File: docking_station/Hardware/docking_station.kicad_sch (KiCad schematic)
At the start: 86 parts, among them IC1 VOM1271T, IC2 VOM1271T, IC3 VOM1271T, IC4 VOM1271T, IC5 VOM1271T, J1 WAGO, J2 XT60, J3 Conn_01x05_Pin, J5 SUPPLY+, J6 SUPPLY-, K1 RELPOL R40N-3021-85-1024, Q1 SIDR392DP-T1-GE3, Q10 2N7002K, Q11 2N7002K, Q12 2N7002K, Q2 SIDR392DP-T1-GE3, Q3 SIDR392DP-T1-GE3, Q4 SIDR392DP-T1-GE3, Q5 SIDR392DP-T1-GE3, Q6 SIDR392DP-T1-GE3, Q7 SIDR392DP-T1-GE3, Q8 SIDR392DP-T1-GE3, Q9 SIDR392DP-T1-GE3, U1 LTC4357MS8, U2 ACS712xLCTR-20A, U3 L78L05AB, U4 LMV321IYLT, U5 MCP6561T-E/OT, U6 MCP6561T-E/OT

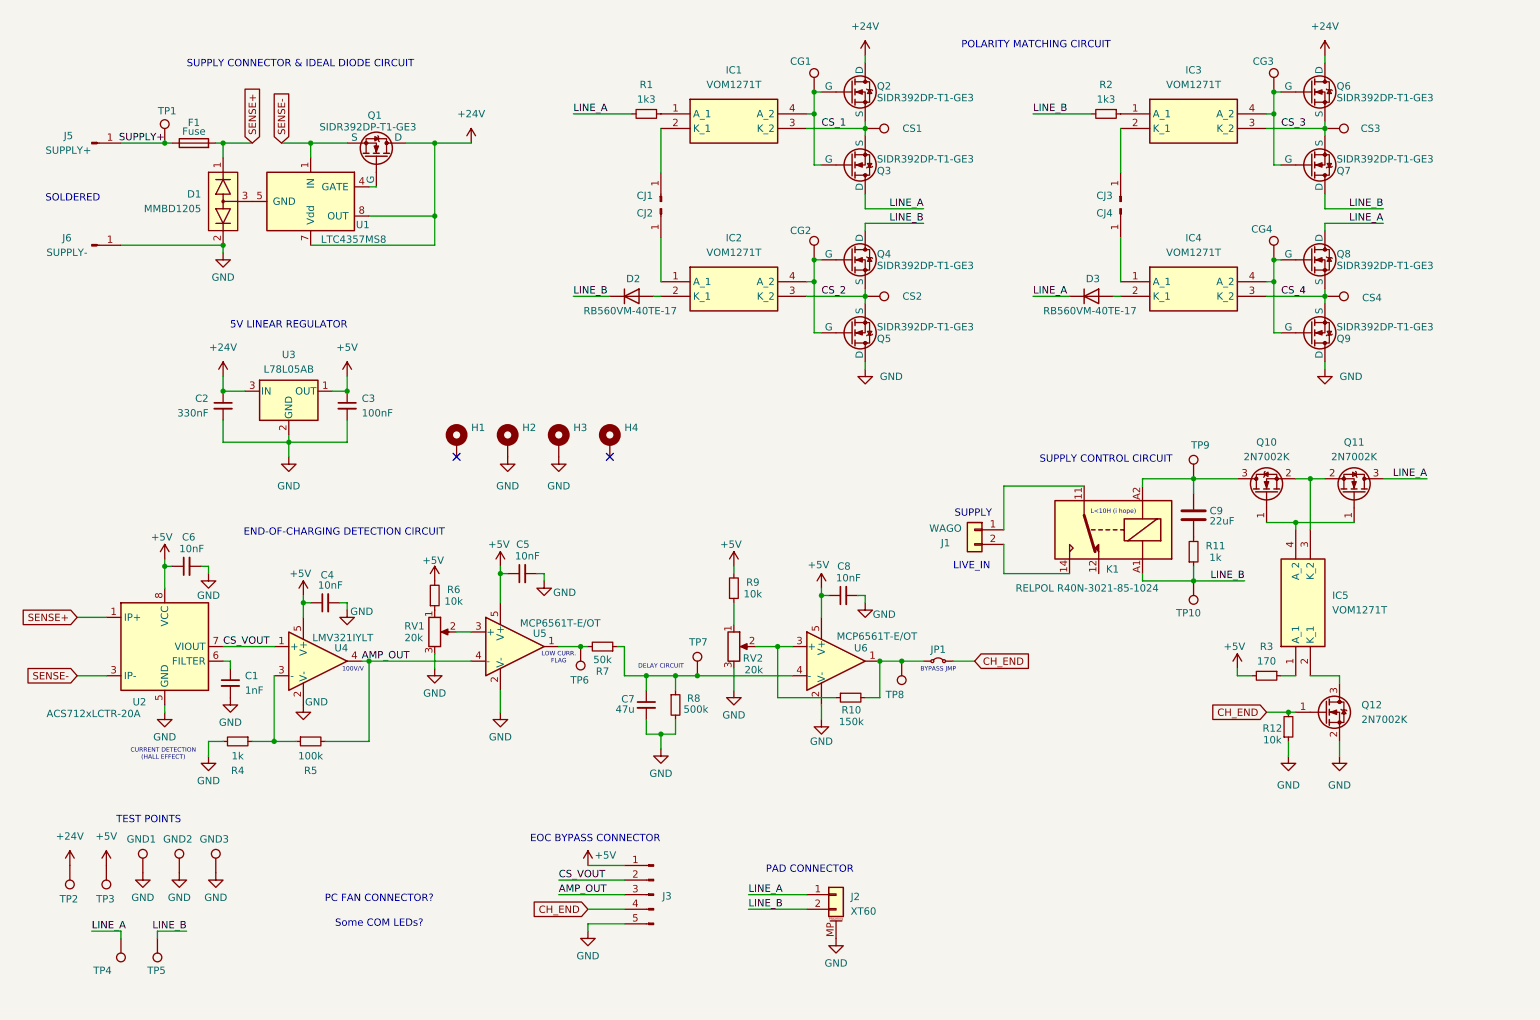
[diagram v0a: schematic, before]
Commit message: Readability update begin
Added LEDs
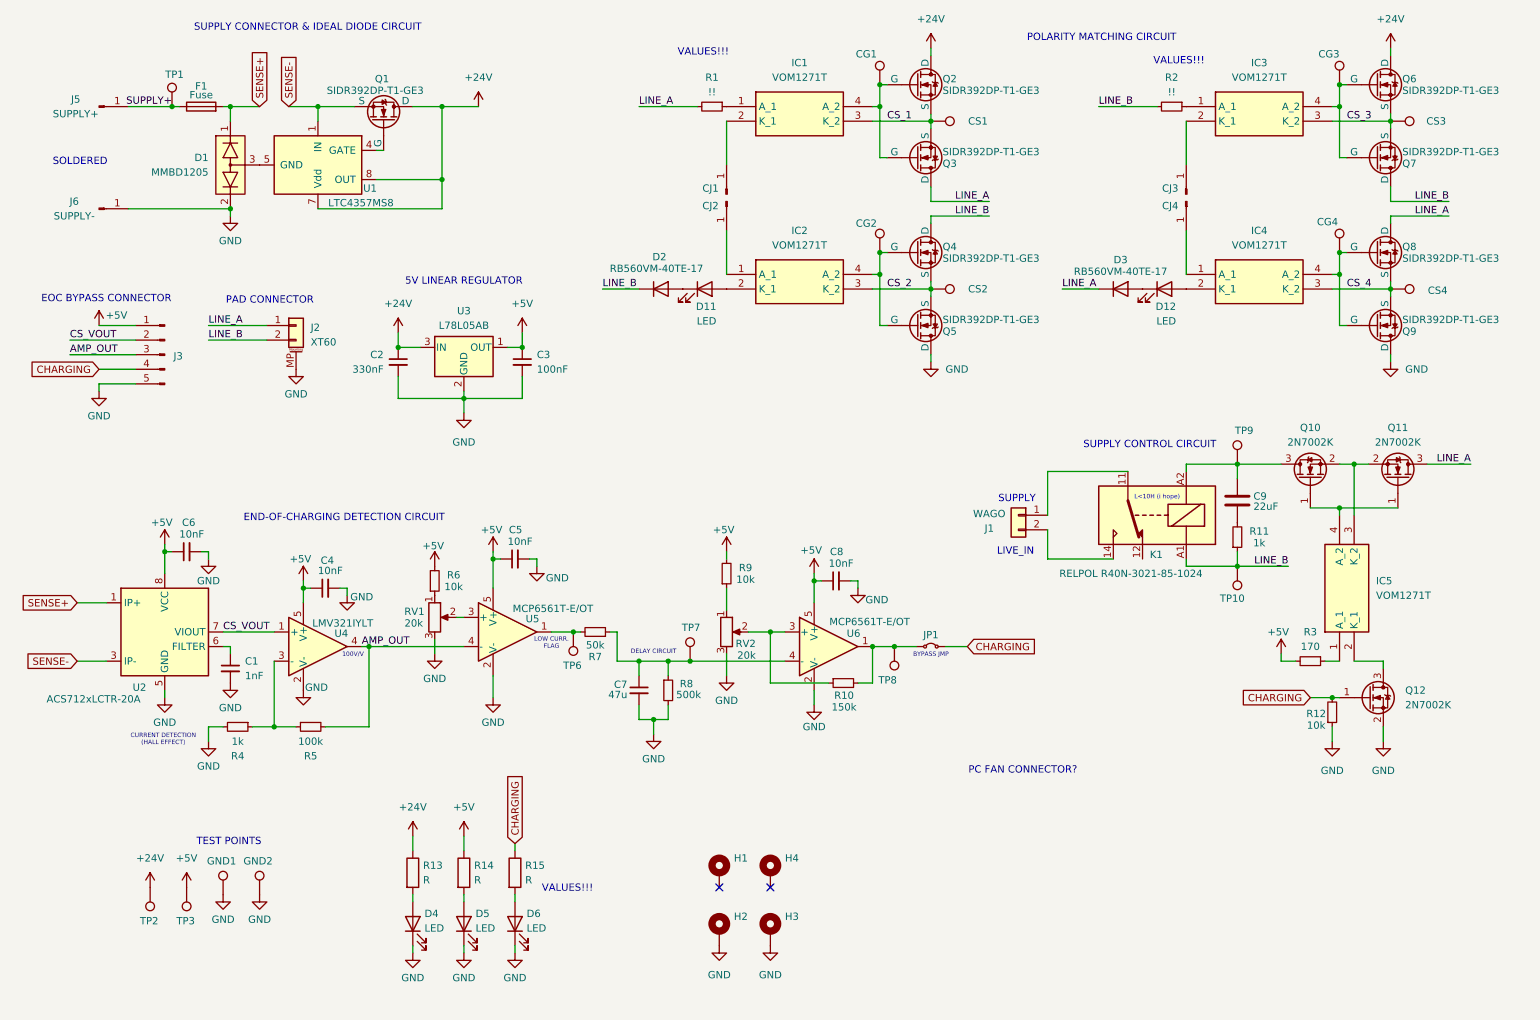
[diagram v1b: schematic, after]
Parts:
- removed GND3: TestPoint, TestPoint:TestPoint_Bridge_Pitch3.81mm_Drill1.3mm, symbol Connector:TestPoint
- removed TP4, TP5: TestPoint, TestPoint:TestPoint_Pad_D2.0mm, symbol Connector:TestPoint
- added D11, D12, D4, D5, D6: LED, LED_SMD:LED_0805_2012Metric, symbol Device:LED
- added R13, R14, R15: R, Resistor_SMD:R_0805_2012Metric, symbol Device:R
- R1, R2: value 1k3 -> !!
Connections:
- net +24V: now also R13.1
- net +5V: now also R14.1
- net GND: now also D4.1 (K), D5.1 (K), D6.1 (K)
- net at D3.2 (A): now also D12.1 (K); no longer IC4.2 (K_1)
- net at IC2.2 (K_1): now also D11.2 (A); no longer D2.2 (A)
- net CH_END renamed CHARGING
- net CHARGING: now also R15.1
- new net: D6.2 (A), R15.2
- new net: D5.2 (A), R14.2
- new net: D4.2 (A), R13.2
- new net: D11.1 (K), D2.2 (A)
- new net: D12.2 (A), IC4.2 (K_1)
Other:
- note added: "VALUES!!!"
- note removed: "Some COM LEDs?"
- moved on the sheet: C1, C2, C3, C4, C5, C6, C7, C8, C9, CG1, CG2, CG3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

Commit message: PCB layout, design and BOM complete; pending review
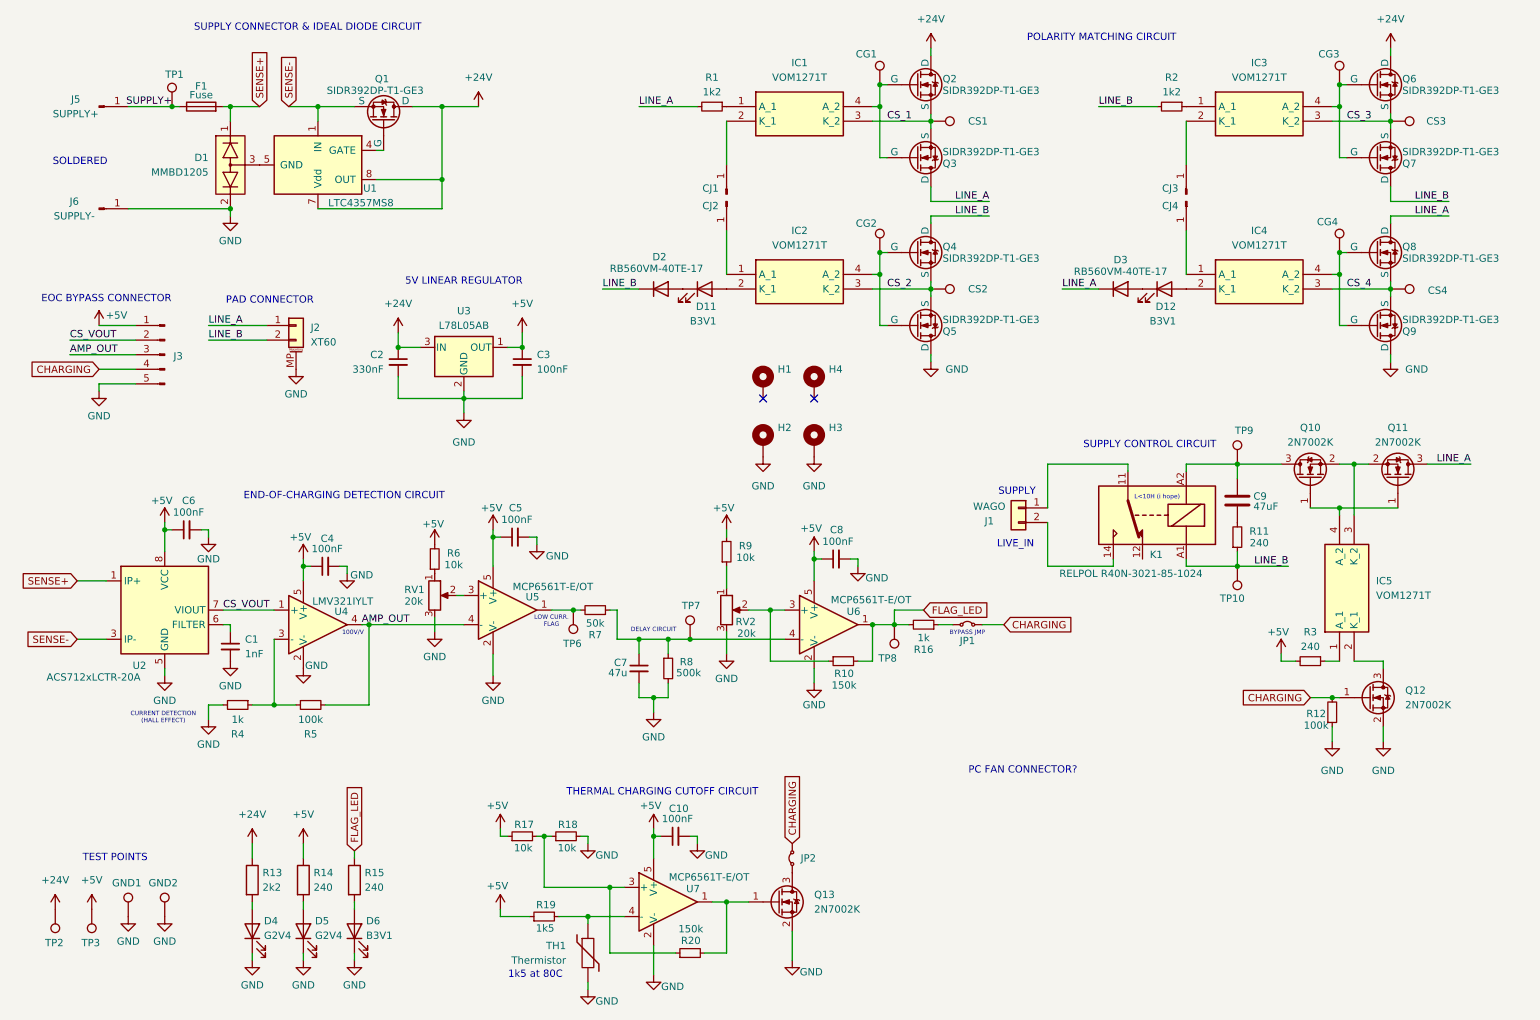
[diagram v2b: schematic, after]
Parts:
- added C10: 100nF, Capacitor_SMD:C_0805_2012Metric, symbol Device:C_Small
- added JP2: Jumper_2_Small_Bridged, Jumper:SolderJumper-2_P1.3mm_Bridged2Bar_RoundedPad1.0x1.5mm, symbol Jumper:Jumper_2_Small_Bridged
- added Q13: 2N7002K, Package_TO_SOT_SMD:SOT-23, symbol Transistor_FET:2N7002K
- added R16: 1k, Resistor_SMD:R_0402_1005Metric, symbol Device:R_Small
- added R17, R18: 10k, Resistor_SMD:R_0402_1005Metric, symbol Device:R_Small
- added R19: 1k5, Resistor_SMD:R_0402_1005Metric, symbol Device:R_Small
- added R20: 150k, Resistor_SMD:R_0402_1005Metric, symbol Device:R_Small
- added TH1: Thermistor, Resistor_THT:R_Axial_DIN0204_L3.6mm_D1.6mm_P2.54mm_Vertical, symbol Device:Thermistor
- added U7: MCP6561T-E/OT, Package_TO_SOT_SMD:SOT-23-5, symbol Comparator:MCP6561-OT
- C4, C5, C6, C8: value 10nF -> 100nF
- C9: value 22uF -> 47uF
- D11, D12, D6: value LED -> B3V1
- D4, D5: value LED -> G2V4
- J2: footprint Connector_AMASS:AMASS_XT60PW-F_1x02_P7.20mm_Horizontal -> firo_footprints:AMASS_XT60PW-F-MP
- R1, R2: value !! -> 1k2
- R11: value 1k -> 240; footprint Resistor_SMD:R_1206_3216Metric -> Resistor_SMD:R_0805_2012Metric
- R12: value 10k -> 100k
- R13: value R -> 2k2; footprint Resistor_SMD:R_0805_2012Metric -> Resistor_SMD:R_1206_3216Metric
- R14, R15: value R -> 240
- R3: value 170 -> 240
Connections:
- net +5V: now also C10.1, R17.1, R19.1, U7.5 (V+)
- net CHARGING: now also JP2.2 (B); no longer R15.1
- net GND: now also C10.2, Q13.2 (S), R18.2, TH1.2, U7.2 (V-)
- net FLAG_LED: now reaches R10.2, TP8.1, U6.1
- net FLAG_LED: now also R15.1, R16.2; no longer JP1.1 (A)
- new net: R19.2, TH1.1, U7.4 (-)
- new net: JP1.1 (A), R16.1
- new net: Q13.1 (G), R20.2, U7.1
- new net: JP2.1 (A), Q13.3 (D)
- new net: R17.2, R18.1, R20.1, U7.3 (+)
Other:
- note added: "1k5 at 80C"
- note added: "THERMAL CHARGING CUTOFF CIRCUIT"
- note removed: "VALUES!!!"
- title: Charging Station Controller for FIRO rover -> Charging Station Controller for FIRO 2.1 rover
- moved on the sheet: C1, C4, C5, C6, C7, C8, D4, D5, D6, GND1, GND2, H1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
